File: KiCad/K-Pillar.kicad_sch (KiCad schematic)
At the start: 6 parts, among them J1 I2COut, J2 Kaypad, M1 Motor_DC, Q1 IRLZ34N, U1 ATmega328-P, U2 L7805

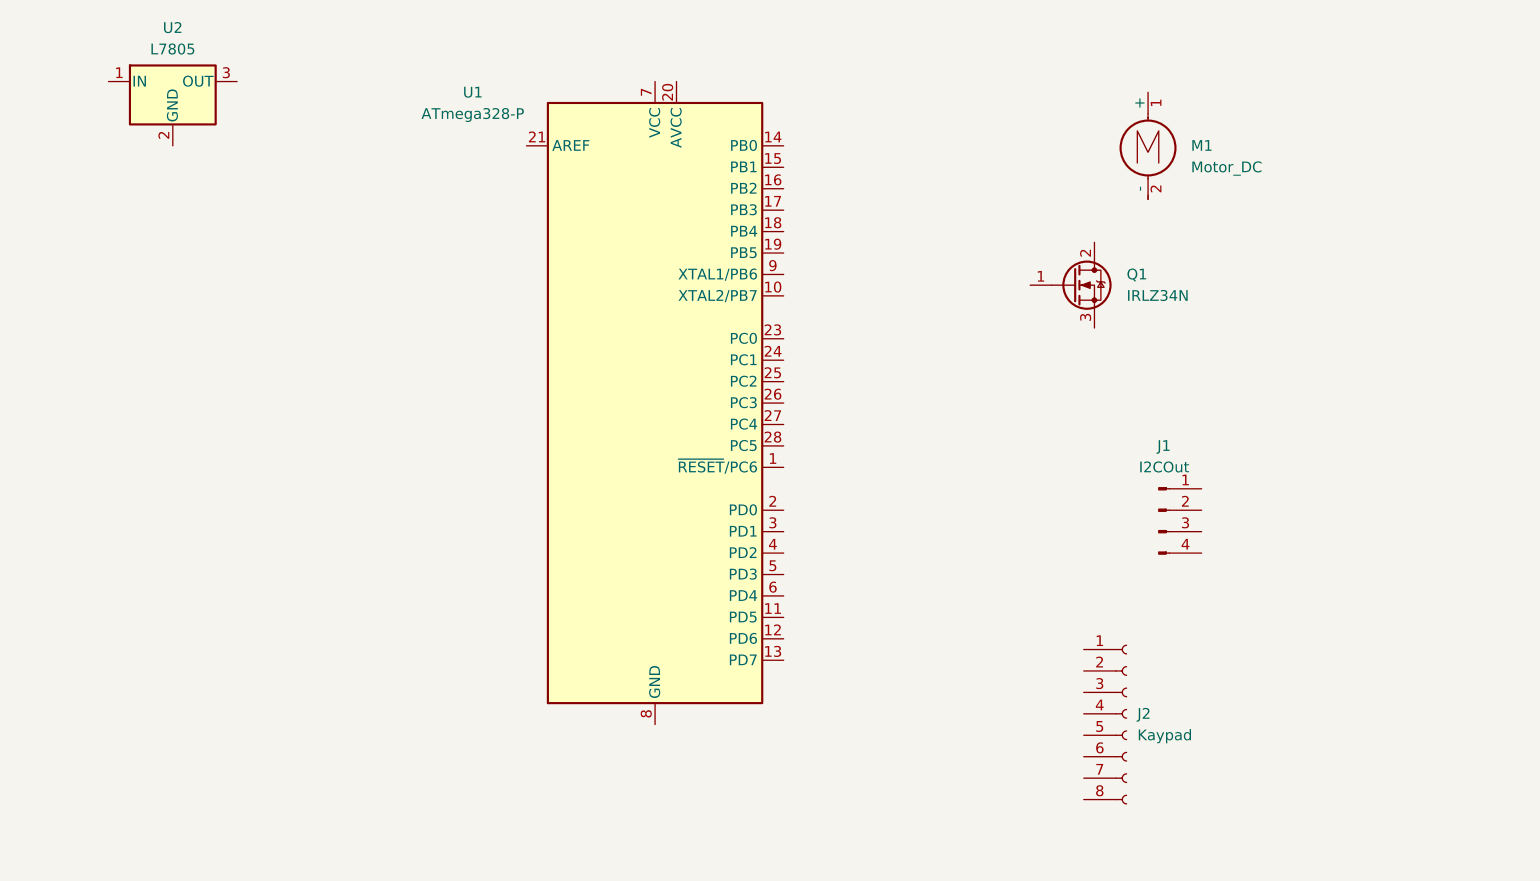
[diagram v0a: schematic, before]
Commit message: płytka zrobiona można na narty
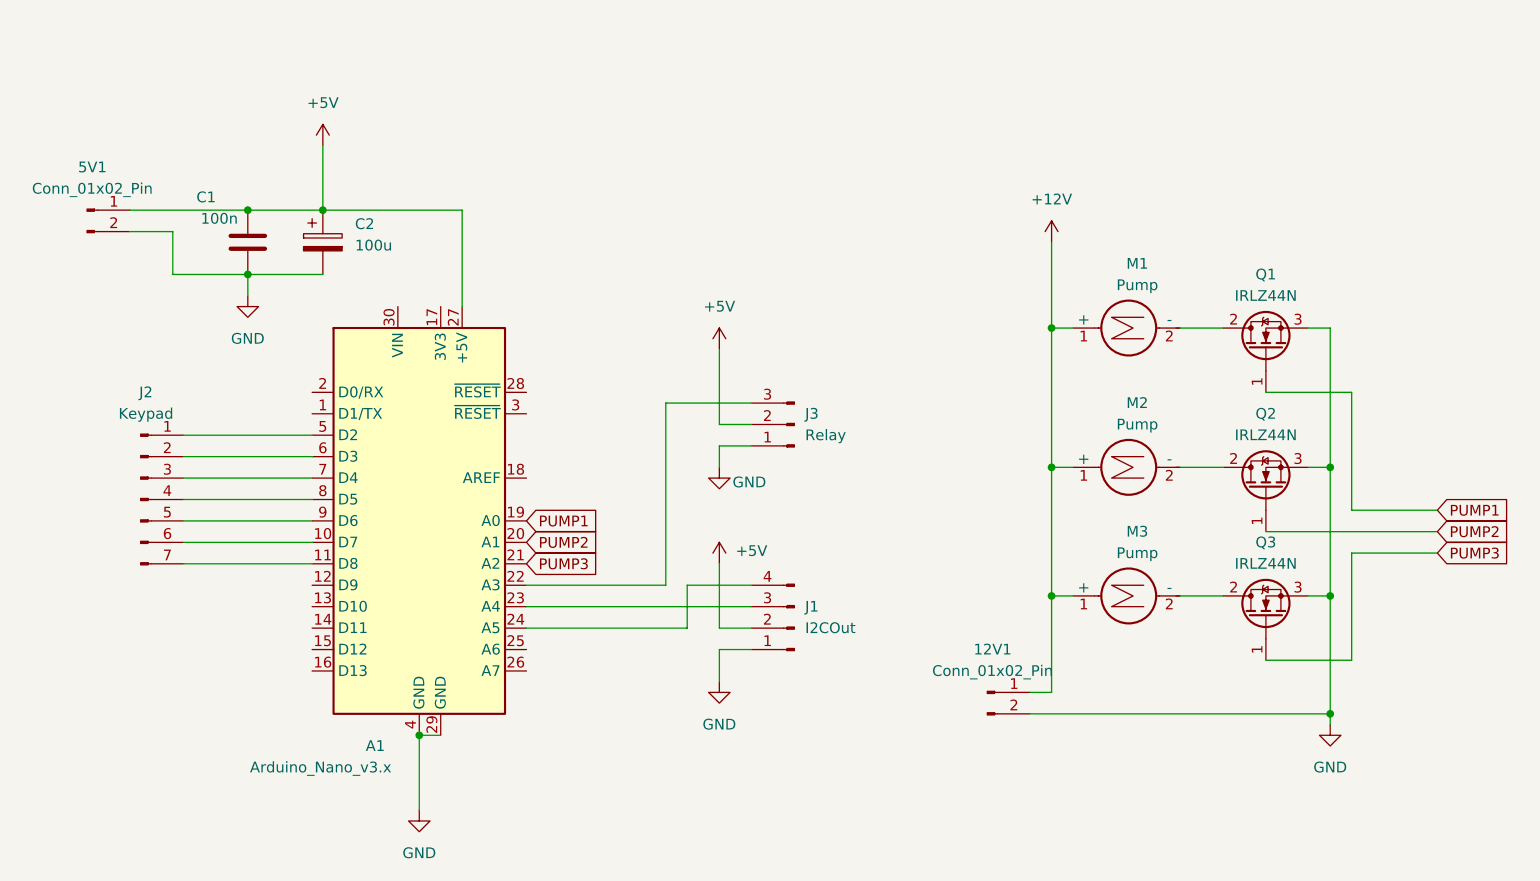
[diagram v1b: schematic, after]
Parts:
- removed J2: Kaypad, symbol Connector:Conn_01x08_Socket
- removed U1: ATmega328-P, Package_DIP:DIP-28_W7.62mm, symbol MCU_Microchip_ATmega:ATmega328-P
- removed U2: L7805, symbol Regulator_Linear:L7805
- added 12V1, 5V1: Conn_01x02_Pin, Connector_PinHeader_2.54mm:PinHeader_1x02_P2.54mm_Vertical, symbol Connector:Conn_01x02_Pin
- added A1: Arduino_Nano_v3.x, Module:Arduino_Nano, symbol MCU_Module:Arduino_Nano_v3.x
- added C1: 100n, Capacitor_SMD:C_0805_2012Metric_Pad1.18x1.45mm_HandSolder, symbol Device:C
- added C2: 100u, Capacitor_THT:CP_Radial_D5.0mm_P2.50mm, symbol Device:C_Polarized
- added J2: Keypad, Connector_PinHeader_2.54mm:PinHeader_1x07_P2.54mm_Vertical, symbol Connector:Conn_01x07_Pin
- added J3: Relay, Connector_PinHeader_2.54mm:PinHeader_1x03_P2.54mm_Vertical, symbol Connector:Conn_01x03_Pin
- added M2, M3: Pump, TerminalBlock_4Ucon:TerminalBlock_4Ucon_1x02_P3.50mm_Horizontal, symbol Motor:Motor_DC
- added Q2, Q3: IRLZ44N, Package_TO_SOT_THT:TO-220-3_Vertical, symbol Transistor_FET:IRLZ34N
- J1: footprint (none) -> Connector_PinHeader_2.54mm:PinHeader_1x04_P2.54mm_Vertical
- M1: value Motor_DC -> Pump; footprint (none) -> TerminalBlock_4Ucon:TerminalBlock_4Ucon_1x02_P3.50mm_Horizontal
- Q1: value IRLZ34N -> IRLZ44N
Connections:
- net GND: now reaches J1.1 (Pin_1)
- net GND: now also Q1.3 (S), 12V1.2 (Pin_2), 5V1.2 (Pin_2), A1.29 (GND), A1.4 (GND), C1.1, C2.2, J3.1 (Pin_1), Q2.3 (S), Q3.3 (S)
- net +5V: now reaches J1.2 (Pin_2)
- net +5V: now also 5V1.1 (Pin_1), A1.27 (+5V), C1.2, C2.1, J3.2 (Pin_2)
- net at J1.3 (Pin_3): now also A1.23 (A4)
- net at J1.4 (Pin_4): now also A1.24 (A5)
- net +12V: now reaches M1.1 (+)
- net +12V: now also 12V1.1 (Pin_1), M2.1 (+), M3.1 (+)
- net at M1.2 (-): now also Q1.2 (D)
- net PUMP1: now reaches Q1.1 (G)
- net PUMP1: now also A1.19 (A0)
- new net: M3.2 (-), Q3.2 (D)
- new net: A1.10 (D7), J2.6 (Pin_6)
- new net: A1.11 (D8), J2.7 (Pin_7)
- new net: A1.22 (A3), J3.3 (Pin_3)
- new net: A1.5 (D2), J2.1 (Pin_1)
- new net: A1.6 (D3), J2.2 (Pin_2)
- new net: A1.7 (D4), J2.3 (Pin_3)
- new net: A1.8 (D5), J2.4 (Pin_4)
- new net: A1.9 (D6), J2.5 (Pin_5)
- new net: M2.2 (-), Q2.2 (D)
- new net PUMP2: A1.20 (A1), Q2.1 (G)
- new net PUMP3: A1.21 (A2), Q3.1 (G)
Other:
- moved on the sheet: J1, M1, Q1
